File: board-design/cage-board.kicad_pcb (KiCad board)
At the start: 2 copper layers, 127 x 152.4 mm, 34 parts, among them J1 Jack-DC, J10 73131-0240, J11 73131-0240, J12 73131-0240, J13 Conn_01x02, J14 Conn_01x02, J15 Conn_02x13_test_points, J2 Conn_02x17_Ribbon, J3 TB002-500-03BE, J4 73131-0240, J5 73131-0240, J6 73131-0240, J7 TB002-500-03BE, J8 73131-0240, J9 TB002-500-03BE, Q1 BD139, Q2 BD139, U1 74LS06, U3 ERJ-UP8F6200V, U4 ERJ-UP8F6200V

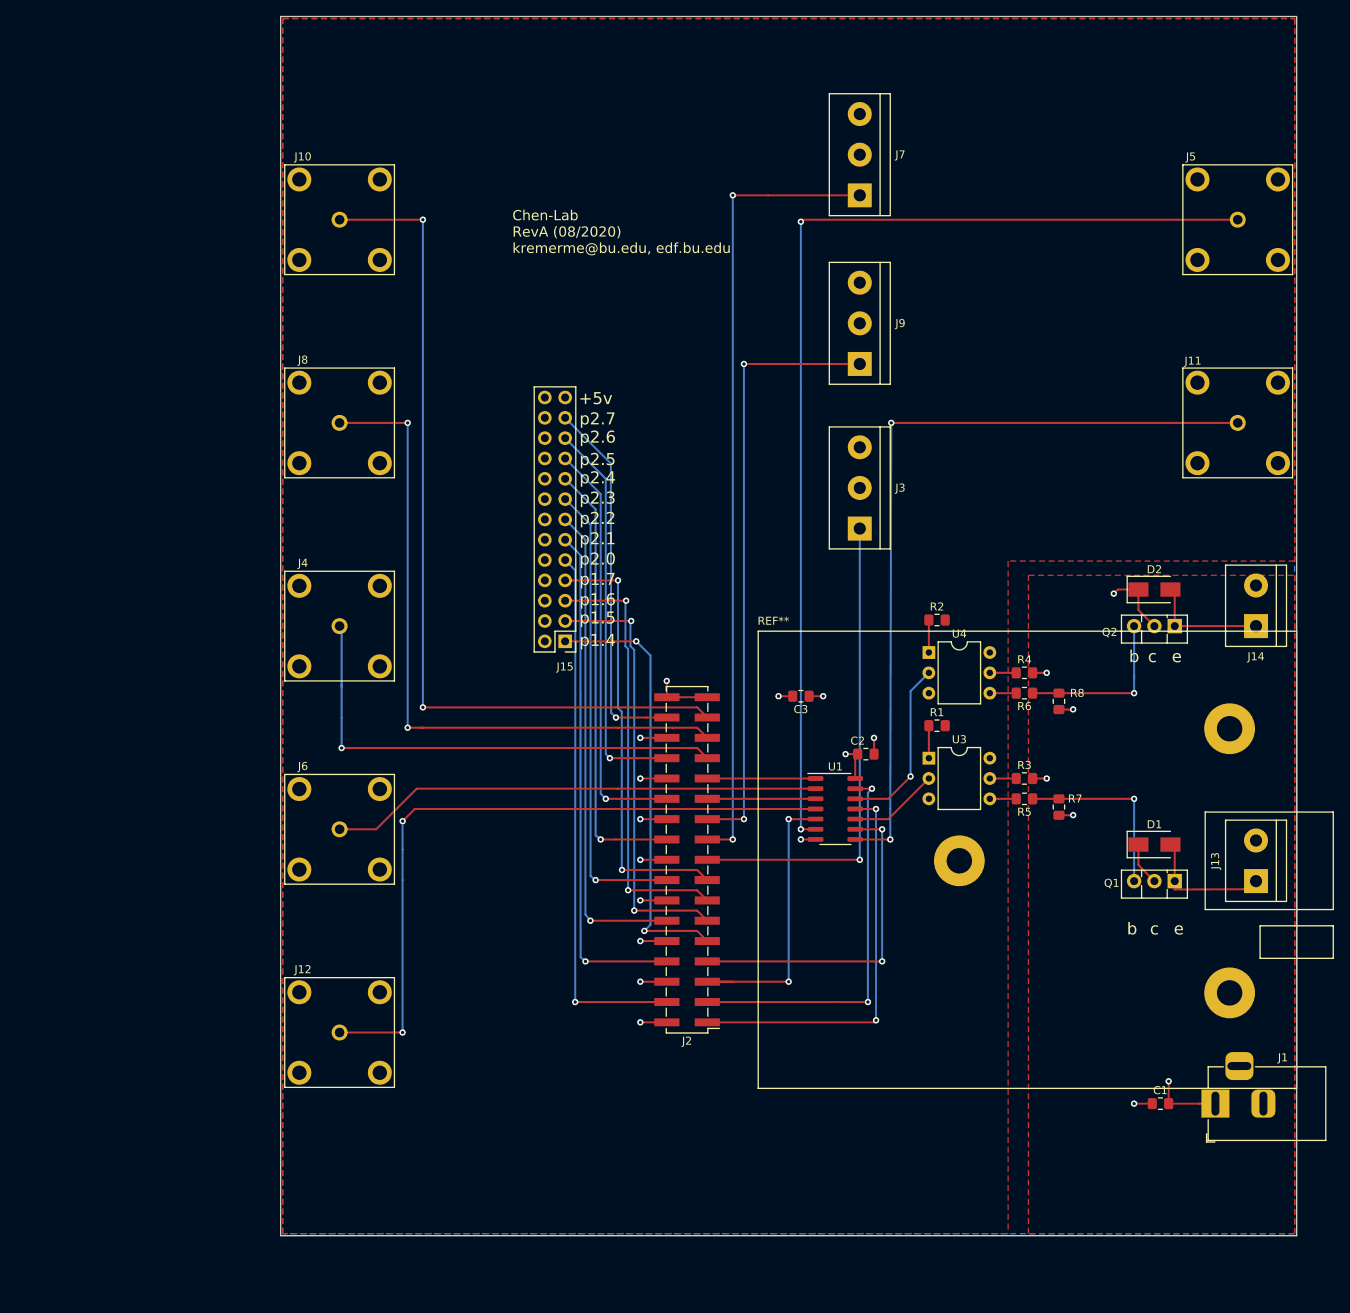
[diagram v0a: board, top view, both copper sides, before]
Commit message: working on resizing board
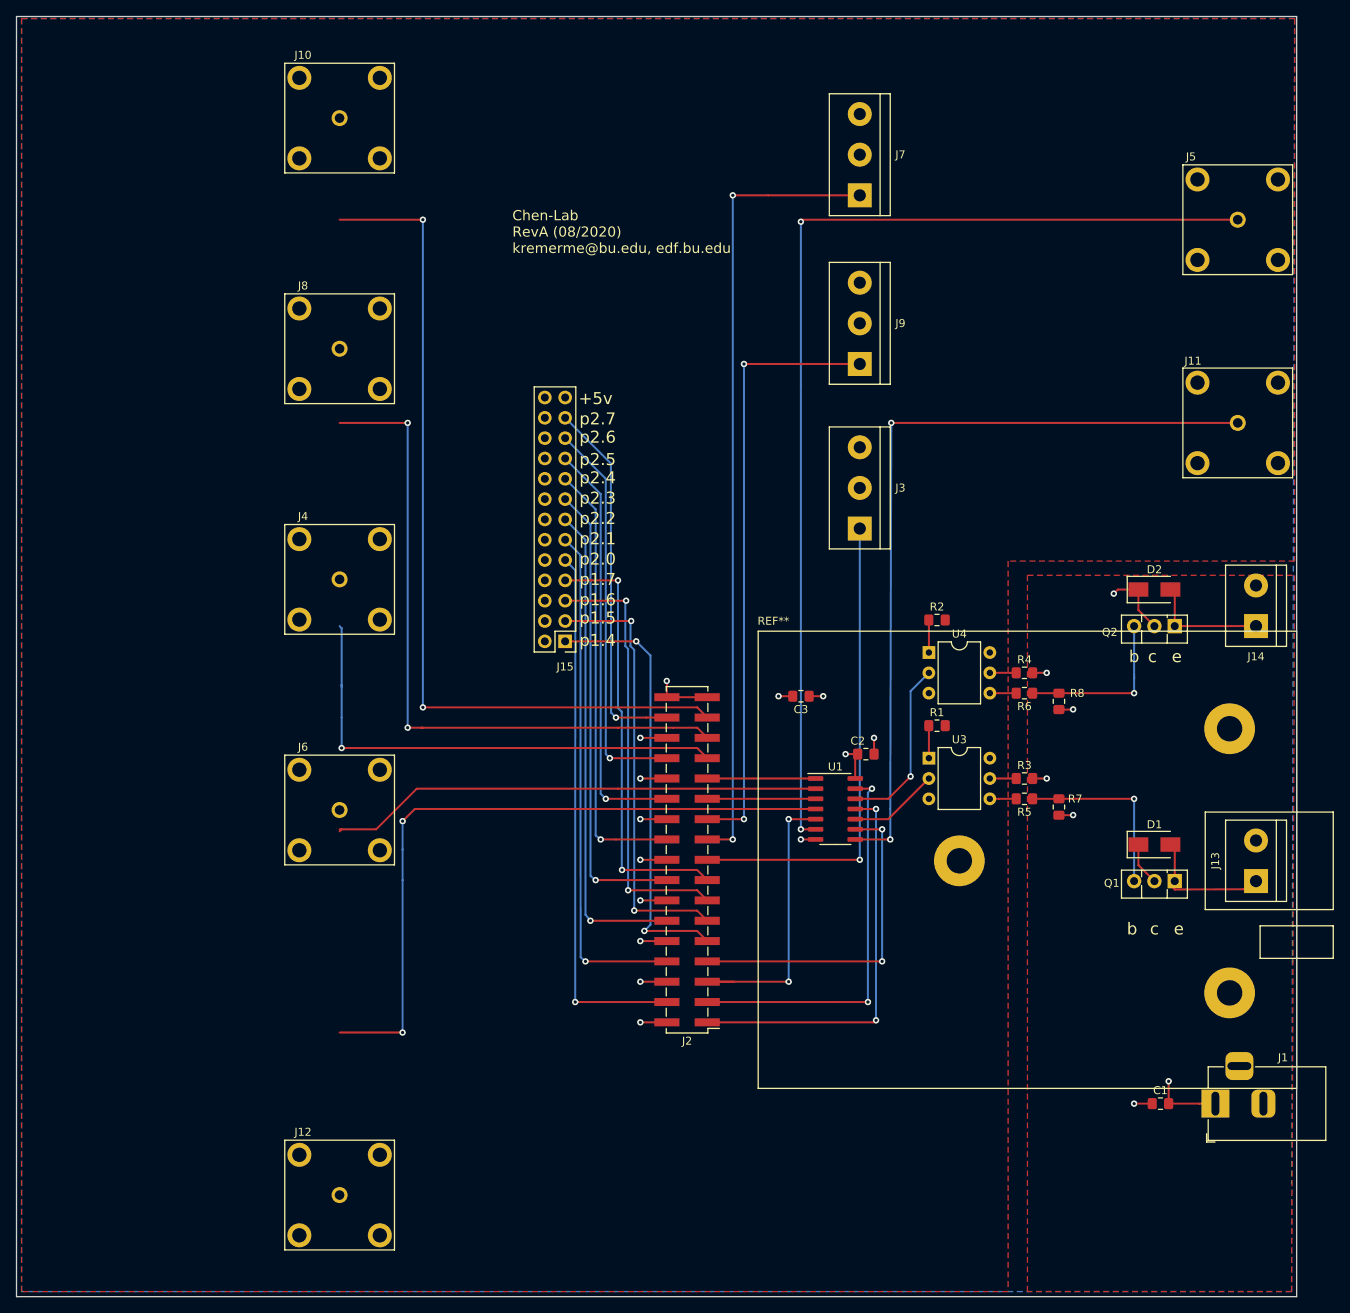
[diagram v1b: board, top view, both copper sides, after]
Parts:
- moved J12 20.3 mm to (83.6, 147.3)
- moved J10 12.7 mm to (83.6, 12.7)
- moved J8 9.27 mm to (83.6, 41.5)
- moved J4 5.84 mm to (83.6, 70.4)
- moved J6 2.41 mm to (83.6, 99.2)
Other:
- board size 127 x 152.4 mm -> 160 x 160 mm
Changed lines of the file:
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@@
-(kicad_pcb (version 20171130) (host pcbnew 5.1.6)
+(kicad_pcb (version 20171130) (host pcbnew 5.1.5+dfsg1-2build2)
   (general
     (thickness 1.6)
@@
   )
   (module chen-lab:BNC-Chen (layer F.Cu)
-    (at 83.566 76.2)
+    (at 83.566 70.358)
     (fp_text reference J4 (at -4.572 -7.874) (layer F.SilkS)
       (effects (font (size 1 1) (thickness 0.15)))
@@
   )
   (module chen-lab:BNC-Chen (layer F.Cu)
-    (at 83.566 101.6)
+    (at 83.566 99.187)
     (fp_text reference J6 (at -4.572 -7.874) (layer F.SilkS)
       (effects (font (size 1 1) (thickness 0.15)))
@@
   )
   (module chen-lab:BNC-Chen (layer F.Cu)
-    (at 83.566 50.8)
+    (at 83.566 41.529)
     (fp_text reference J8 (at -4.572 -7.874) (layer F.SilkS)
       (effects (font (size 1 1) (thickness 0.15)))
@@
   )
   (module chen-lab:BNC-Chen (layer F.Cu)
-    (at 83.566 25.4)
+    (at 83.566 12.7)
     (fp_text reference J10 (at -4.572 -7.874) (layer F.SilkS)
       (effects (font (size 1 1) (thickness 0.15)))
@@
   )
   (module chen-lab:BNC-Chen (layer F.Cu)
-    (at 83.566 127)
+    (at 83.566 147.32)
     (fp_text reference J12 (at -4.572 -7.874) (layer F.SilkS)
       (effects (font (size 1 1) (thickness 0.15)))
@@
     (effects (font (size 1.27 1.27) (thickness 0.1778)) (justify left))
   )
-  (gr_line (start 76.2 0) (end 76.2 152.4) (layer Edge.Cuts) (width 0.127))
-  (gr_line (start 203.2 0) (end 203.2 152.4) (layer Edge.Cuts) (width 0.127))
-  (gr_line (start 76.2 0) (end 203.2 0) (layer Edge.Cuts) (width 0.127))
-  (gr_line (start 76.2 152.4) (end 203.2 152.4) (layer Edge.Cuts) (width 0.127))
+  (gr_line (start 43.18 0) (end 43.18 160.02) (layer Edge.Cuts) (width 0.127))
+  (gr_line (start 203.2 0) (end 203.2 160.02) (layer Edge.Cuts) (width 0.127))
+  (gr_line (start 43.18 0) (end 203.2 0) (layer Edge.Cuts) (width 0.127))
+  (gr_line (start 43.18 160.02) (end 203.2 160.02) (layer Edge.Cuts) (width 0.127))
   (segment (start 183.42 74.2) (end 183.42 71.628) (width 0.25) (layer F.Cu) (net 1))
   (segment (start 185.42 76.2) (end 183.42 74.2) (width 0.25) (layer F.Cu) (net 1))
@@
   (via (at 152.4 102.87) (size 0.8) (drill 0.4) (layers F.Cu B.Cu) (net 30))
   (segment (start 143.067 99.06) (end 142.24 99.06) (width 0.25) (layer F.Cu) (net 31))
-  (segment (start 83.566 127) (end 91.44 127) (width 0.25) (layer F.Cu) (net 31))
   (segment (start 142.24 99.06) (end 120.015 99.06) (width 0.25) (layer F.Cu) (net 31))
-  (segment (start 91.44 107.95) (end 91.44 104.14) (width 0.25) (layer B.Cu) (net 31))
-  (segment (start 91.44 127) (end 91.44 107.95) (width 0.25) (layer B.Cu) (net 31))
-  (via (at 91.44 127) (size 0.8) (drill 0.4) (layers F.Cu B.Cu) (net 31))
   (via (at 91.44 100.584) (size 0.8) (drill 0.4) (layers F.Cu B.Cu) (net 31))
   (segment (start 92.964 99.06) (end 91.44 100.584) (width 0.25) (layer F.Cu) (net 31))
   (segment (start 93.472 99.06) (end 92.964 99.06) (width 0.25) (layer F.Cu) (net 31))
   (segment (start 120.142 99.06) (end 93.472 99.06) (width 0.25) (layer F.Cu) (net 31))
+  (segment (start 83.566 127) (end 91.44 127) (width 0.25) (layer F.Cu) (net 31))
+  (via (at 91.44 127) (size 0.8) (drill 0.4) (layers F.Cu B.Cu) (net 31))
+  (segment (start 91.44 127) (end 91.44 107.95) (width 0.25) (layer B.Cu) (net 31))
+  (segment (start 91.44 107.95) (end 91.44 104.14) (width 0.25) (layer B.Cu) (net 31))
   (segment (start 91.44 100.584) (end 91.44 104.14) (width 0.25) (layer B.Cu) (net 31))
   (segment (start 170.198 97.79) (end 173.482 97.79) (width 0.25) (layer F.Cu) (net 32))
@@
     (polygon
       (pts
-        (xy 202.946 68.072) (xy 167.132 68.072) (xy 167.132 152.146) (xy 76.454 152.146) (xy 76.454 0.254)
+        (xy 202.946 68.072) (xy 167.132 68.072) (xy 167.132 159.385) (xy 43.815 159.385) (xy 43.815 0.254)
         (xy 202.946 0.254)
       )
@@
     (polygon
       (pts
-        (xy 202.946 152.146) (xy 76.454 152.146) (xy 76.454 0.254) (xy 202.946 0.254)
+        (xy 202.565 159.385) (xy 43.815 159.385) (xy 43.815 0.254) (xy 202.946 0.254)
       )
     )
@@
     (polygon
       (pts
-        (xy 202.946 152.146) (xy 169.672 152.146) (xy 169.672 69.85) (xy 202.946 69.85)
+        (xy 202.565 159.385) (xy 169.545 159.385) (xy 169.545 69.85) (xy 202.946 69.85)
       )
     )
